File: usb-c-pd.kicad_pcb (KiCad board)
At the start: 2 copper layers, 4.5 x 13.4 mm, 52 parts, among them J1 USB_C_Receptacle_USB2.0_14P, J2 Barrel_Jack_Switch, J3 Conn_ARM_SWD_TagConnect_TC203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, Q1 T2N7002AK, U1 CYPD3177-24LQ, U2 STM32C071F8Px, U3 INA180A2, U4 XL1509-3.3

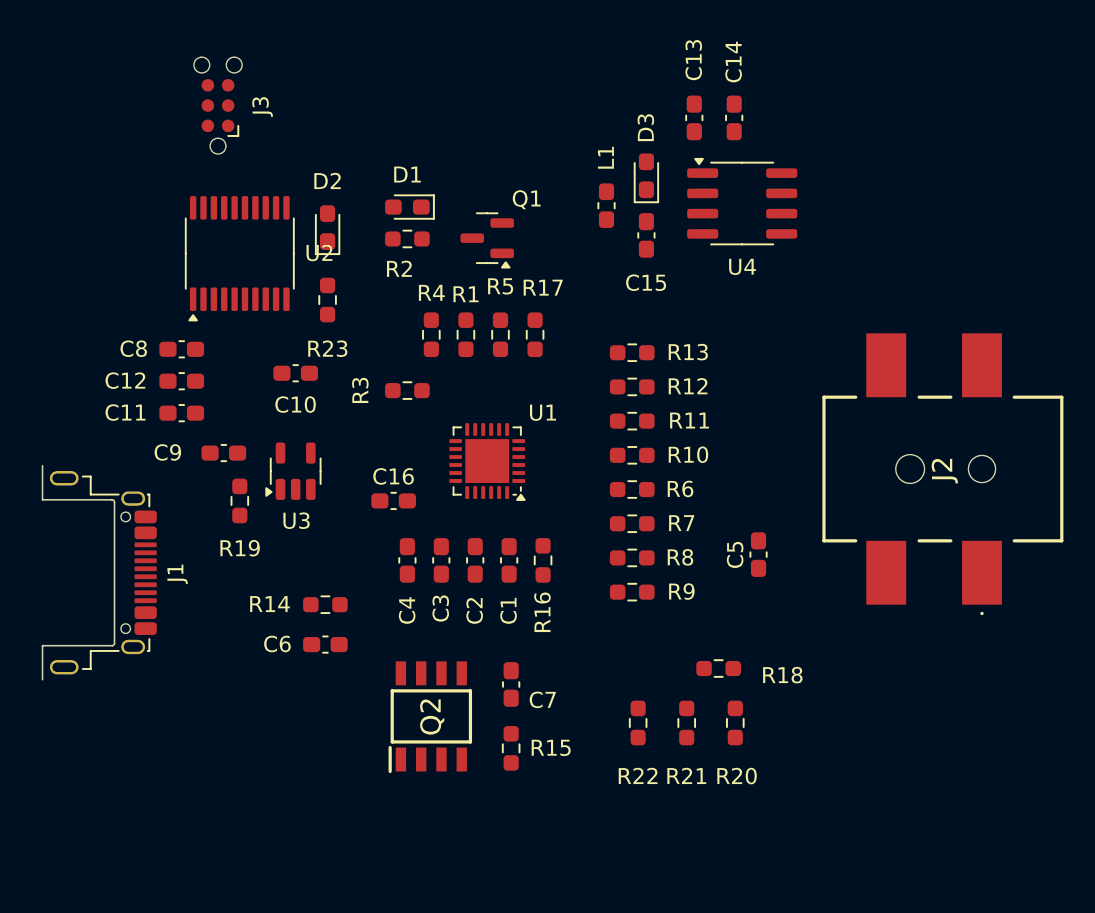
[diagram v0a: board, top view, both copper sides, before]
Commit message: feat: routing
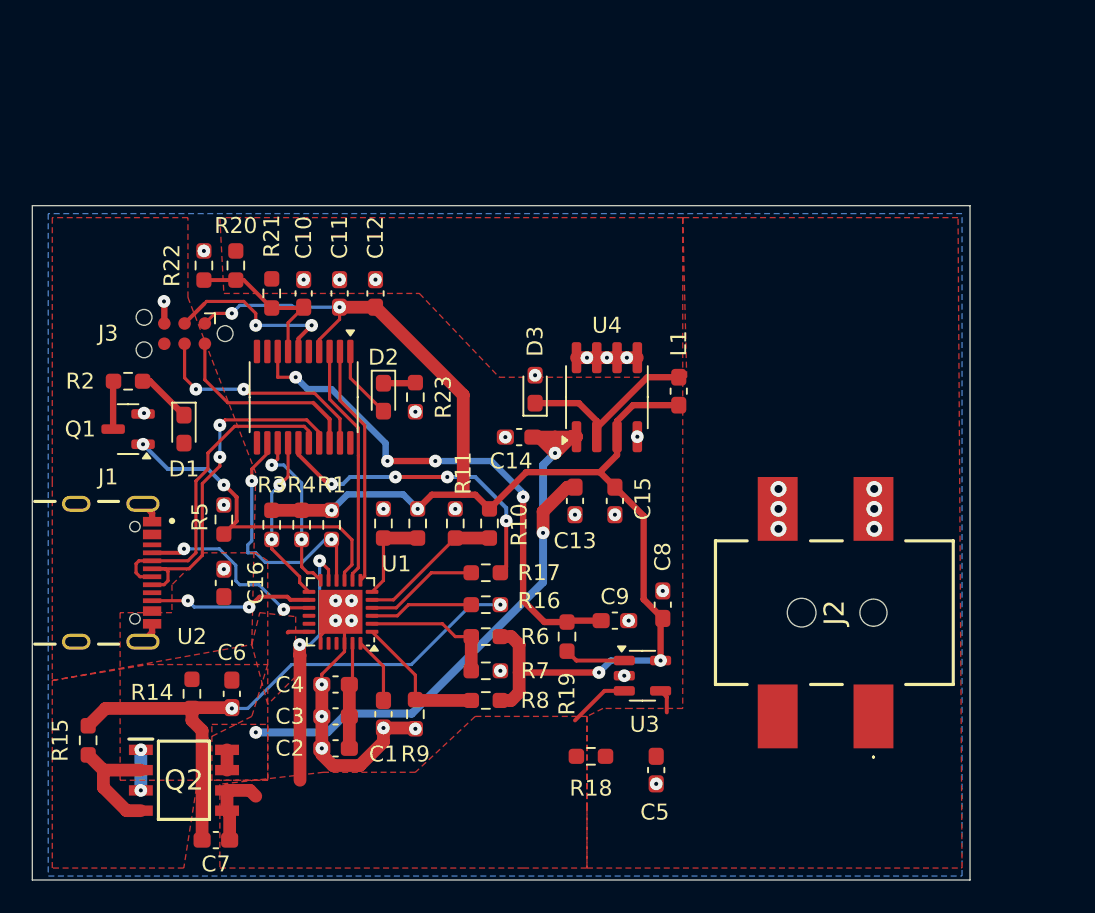
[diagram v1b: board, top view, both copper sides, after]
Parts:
- J1: footprint Connector_USB:USB_C_Receptacle_Amphenol_12401948E412A -> usb-c-pd-lib:GCT_USB4105-GF-A
- moved R20 42.4 mm to (44.2, 66.2)
- moved R22 39.5 mm to (42.2, 66.2)
- moved R21 37.4 mm to (46.5, 68.0)
- moved C8 34.1 mm to (71.0, 87.5), turned to 90 degrees
- moved C9 26.7 mm to (68.0, 88.5), turned to 180 degrees
- moved R15 26.5 mm to (35.0, 96.0)
- moved Q1 25.5 mm to (37.5, 76.5)
- moved U3 25.2 mm to (69.7, 92.0), turned to 0 degrees
- moved C13 25.1 mm to (65.5, 81.0), turned to -90 degrees
- moved C14 24.1 mm to (62.0, 77.0), turned to 180 degrees
- moved R19 22.2 mm to (65.0, 89.5)
- moved C7 20.9 mm to (43.0, 102.2), turned to 180 degrees
- moved R5 20.8 mm to (43.5, 82.2)
- moved D1 19.7 mm to (41.0, 76.5), turned to -90 degrees
- moved R2 19.6 mm to (37.5, 73.5)
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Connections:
- net Net-(J1-CC1) renamed CC1
- net Net-(J1-CC2) renamed CC2
- R1 pad 2: +3V3 -> +3V3 MCU
- R3 pad 1: +3V3 -> +3V3 MCU
- R4 pad 1: +3V3 -> +3V3 MCU
- U2 pad 2: PD_GPIO -> HPI_INT
- U2 pad 3: HPI_INT -> PD_GPIO
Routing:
- net +3V3 MCU: track 0.00 -> 87.7 mm, vias 0 -> 6
- net VBUS: track 0.00 -> 44.3 mm, vias 0 -> 3
- net Net-(C6-Pad2): track 0.00 -> 37.5 mm, vias 0 -> 2
- net AMP_OUT: track 0.00 -> 32.8 mm, vias 0 -> 4
- net GND: track 0.00 -> 27.1 mm, vias 0 -> 39
- net +VBUS_PD: track 0.00 -> 25.1 mm, vias 0 -> 2
- net USB_DP: track 0.00 -> 22.2 mm, vias 0 -> 2
- net Net-(Q1-G): track 0.00 -> 21.3 mm, vias 0 -> 2
- net USB_DM: track 0.00 -> 20.2 mm
- net PD_SAFE: track 0.00 -> 19.7 mm, vias 0 -> 4
- net PD_FLIP: track 0.00 -> 16.3 mm, vias 0 -> 2
- net PD_GPIO: track 0.00 -> 15.2 mm
- net HPI_INT: track 0.00 -> 15.1 mm
- net SWCLK: track 0.00 -> 14.5 mm, vias 0 -> 2
- net SWDIO: track 0.00 -> 12.6 mm
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- added copper zone on F.Cu, net +VBUS_PD
- added copper zone on B.Cu, net GND
- added copper zone on F.Cu, net VBUS
- added copper zone on F.Cu, net VCONN
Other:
- board size 4.5 x 13.4 mm -> 58.8 x 42.2 mm
